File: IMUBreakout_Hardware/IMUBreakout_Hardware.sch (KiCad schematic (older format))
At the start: 6 parts

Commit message: created new part
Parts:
- removed Conn1: Molex_SL_04, MRDT_Connectors:MOLEX_SL_04_Vertical, symbol MRDT_Connectors:Molex_SL_04
- removed Conn2: Molex_SL_08, MRDT_Connectors:MOLEX_SL_08_Vertical, symbol MRDT_Connectors:Molex_SL_08
- added Conn?: Molex_SL_04, MRDT_Connectors:MOLEX_SL_04_Horizontal, symbol MRDT_Connectors:Molex_SL_04
- added U?: Razor_9DOF_Sparkfun, MRDT_Sensors:Razor_9DOF_Sparkfun, symbol MRDT_Sensors:Razor_9DOF_Sparkfun
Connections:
- wire segments 10 -> 18
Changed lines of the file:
@@
 Comment4 ""
 $EndDescr
-$Comp
-L MRDT_Connectors:Molex_SL_04 Conn1
-U 1 1 5C71B502
-P 3530 1646
-F 0 "Conn1" H 3657 1904 60  0000 L CNN
-F 1 "Molex_SL_04" H 3657 1798 60  0000 L CNN
-F 2 "MRDT_Connectors:MOLEX_SL_04_Vertical" H 3530 1646 60  0001 C CNN
-F 3 "" H 3530 1646 60  0001 C CNN
-	1    3530 1646
-	1    0    0    -1
-$EndComp
-Text GLabel 4790 1230 0    50   Input ~ 0
+Text GLabel 4950 1200 0    50   Input ~ 0
 +3V3
-Text GLabel 4790 1430 0    50   Input ~ 0
+Text GLabel 4950 1400 0    50   Input ~ 0
 TX
-Text GLabel 4790 1330 0    50   Input ~ 0
+Text GLabel 4950 1300 0    50   Input ~ 0
 RX
 Wire Notes Line
@@
 Text Notes 3630 680  0    118  ~ 24
 Connections
-Text GLabel 4790 1130 0    50   Input ~ 0
-GND
-$Comp
-L MRDT_Connectors:Molex_SL_08 Conn2
-U 1 1 5C774553
-P 5030 1880
-F 0 "Conn2" H 5157 2338 60  0000 L CNN
-F 1 "Molex_SL_08" H 5157 2232 60  0000 L CNN
-F 2 "MRDT_Connectors:MOLEX_SL_08_Vertical" H 5030 2180 60  0001 C CNN
-F 3 "" H 5030 2180 60  0001 C CNN
-	1    5030 1880
-	1    0    0    -1
-$EndComp
-Wire Wire Line
-	4830 1130 4790 1130
-Wire Wire Line
-	4830 1230 4790 1230
-Wire Wire Line
-	4830 1330 4790 1330
-Wire Wire Line
-	4830 1430 4790 1430
 $Comp
 L Device:R R2
@@
 Wire Notes Line
 	6340 2360 470  2360
+$Comp
+L MRDT_Connectors:Molex_SL_04 Conn?
+U 1 1 5C7ACAF9
+P 5200 1450
+F 0 "Conn?" H 5327 1708 60  0000 L CNN
+F 1 "Molex_SL_04" H 5327 1602 60  0000 L CNN
+F 2 "MRDT_Connectors:MOLEX_SL_04_Horizontal" H 5200 1450 60  0001 C CNN
+F 3 "" H 5200 1450 60  0001 C CNN
+	1    5200 1450
+	1    0    0    -1
+$EndComp
+Text GLabel 4950 1100 0    50   Input ~ 0
+GND
+Wire Wire Line
+	4950 1100 5000 1100
+Wire Wire Line
+	5000 1200 4950 1200
+Wire Wire Line
+	5000 1300 4950 1300
+Wire Wire Line
+	5000 1400 4950 1400
+$Comp
+L MRDT_Sensors:Razor_9DOF_Sparkfun U?
+U 1 1 5C7ACFCA
+P 3600 2000
+F 0 "U?" H 3800 2965 50  0000 C CNN
+F 1 "Razor_9DOF_Sparkfun" H 3800 2874 50  0000 C CNN
+F 2 "MRDT_Sensors:Razor_9DOF_Sparkfun" H 3350 2250 50  0001 C CNN
+F 3 "" H 3350 2250 50  0001 C CNN
+	1    3600 2000
+	1    0    0    -1
+$EndComp
+Text GLabel 3400 1500 0    50   Input ~ 0
++3V3
+Text GLabel 3400 1700 0    50   Input ~ 0
+GND
+Wire Wire Line
+	3500 1450 3500 1500
+Wire Wire Line
+	3400 1500 3500 1500
+Connection ~ 3500 1500
+Wire Wire Line
+	3500 1500 3500 1550
+Wire Wire Line
+	3500 1650 3500 1700
+Wire Wire Line
+	3400 1700 3500 1700
+Connection ~ 3500 1700
+Wire Wire Line
+	3500 1700 3500 1750
+Text GLabel 4150 1450 2    50   Input ~ 0
+RX
+Text GLabel 4150 1550 2    50   Input ~ 0
+TX
+Wire Wire Line
+	4100 1450 4150 1450
+Wire Wire Line
+	4100 1550 4150 1550
 $EndSCHEMATC

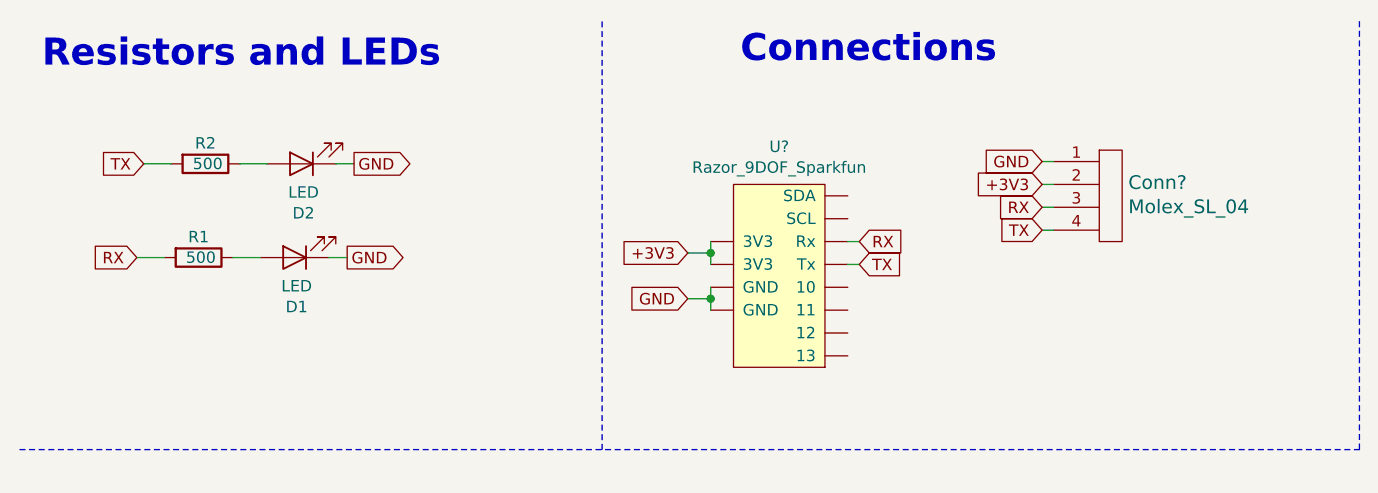
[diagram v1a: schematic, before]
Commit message: PCB Finalzied and Made
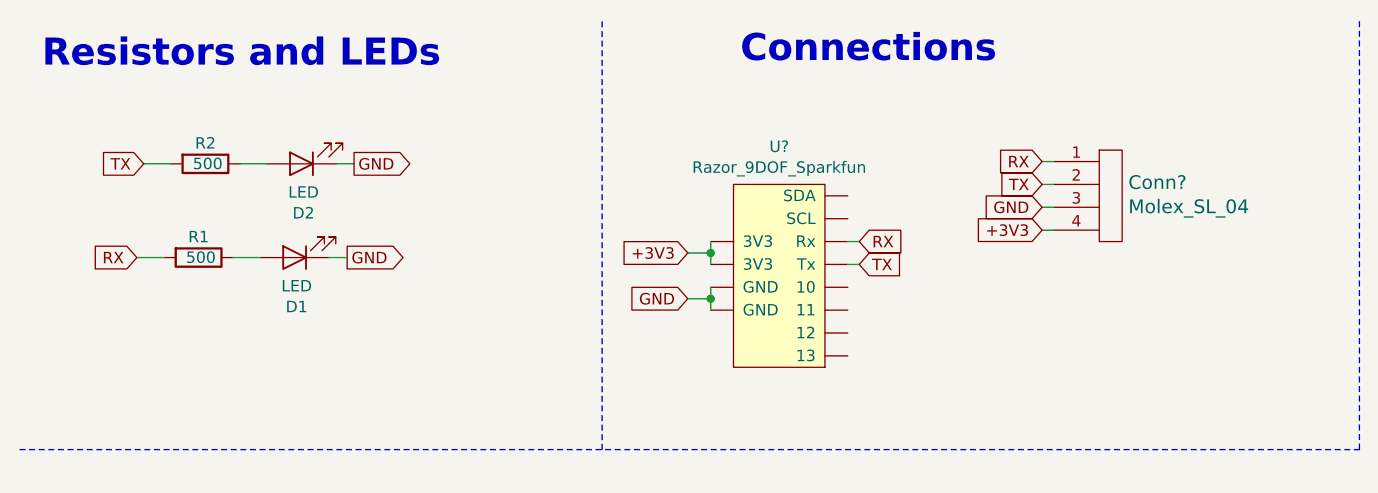
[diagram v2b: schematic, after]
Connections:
- net +3V3: now also Conn?.4; no longer Conn?.2
- net GND: now also Conn?.3; no longer Conn?.1
- net RX: now also Conn?.1; no longer Conn?.3
- net TX: now also Conn?.2; no longer Conn?.4
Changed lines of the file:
@@
 Comment4 ""
 $EndDescr
+Text GLabel 4950 1400 0    50   Input ~ 0
++3V3
 Text GLabel 4950 1200 0    50   Input ~ 0
-+3V3
-Text GLabel 4950 1400 0    50   Input ~ 0
 TX
-Text GLabel 4950 1300 0    50   Input ~ 0
+Text GLabel 4950 1100 0    50   Input ~ 0
 RX
 Wire Notes Line
@@
 	1    0    0    -1
 $EndComp
-Text GLabel 4950 1100 0    50   Input ~ 0
+Text GLabel 4950 1300 0    50   Input ~ 0
 GND
 Wire Wire Line
